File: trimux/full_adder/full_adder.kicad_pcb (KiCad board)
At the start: 2 copper layers, 90.8 x 105.4 mm, 44 parts, among them P1 CONN_01X01, P2 CONN_01X01, P3 CONN_01X01, P4 CONN_01X01, P5 CONN_01X01, P6 CONN_01X03, U1 trimux, U2 trimux, U3 trimux, U4 trimux, U5 trimux, U6 trimux, U7 trimux

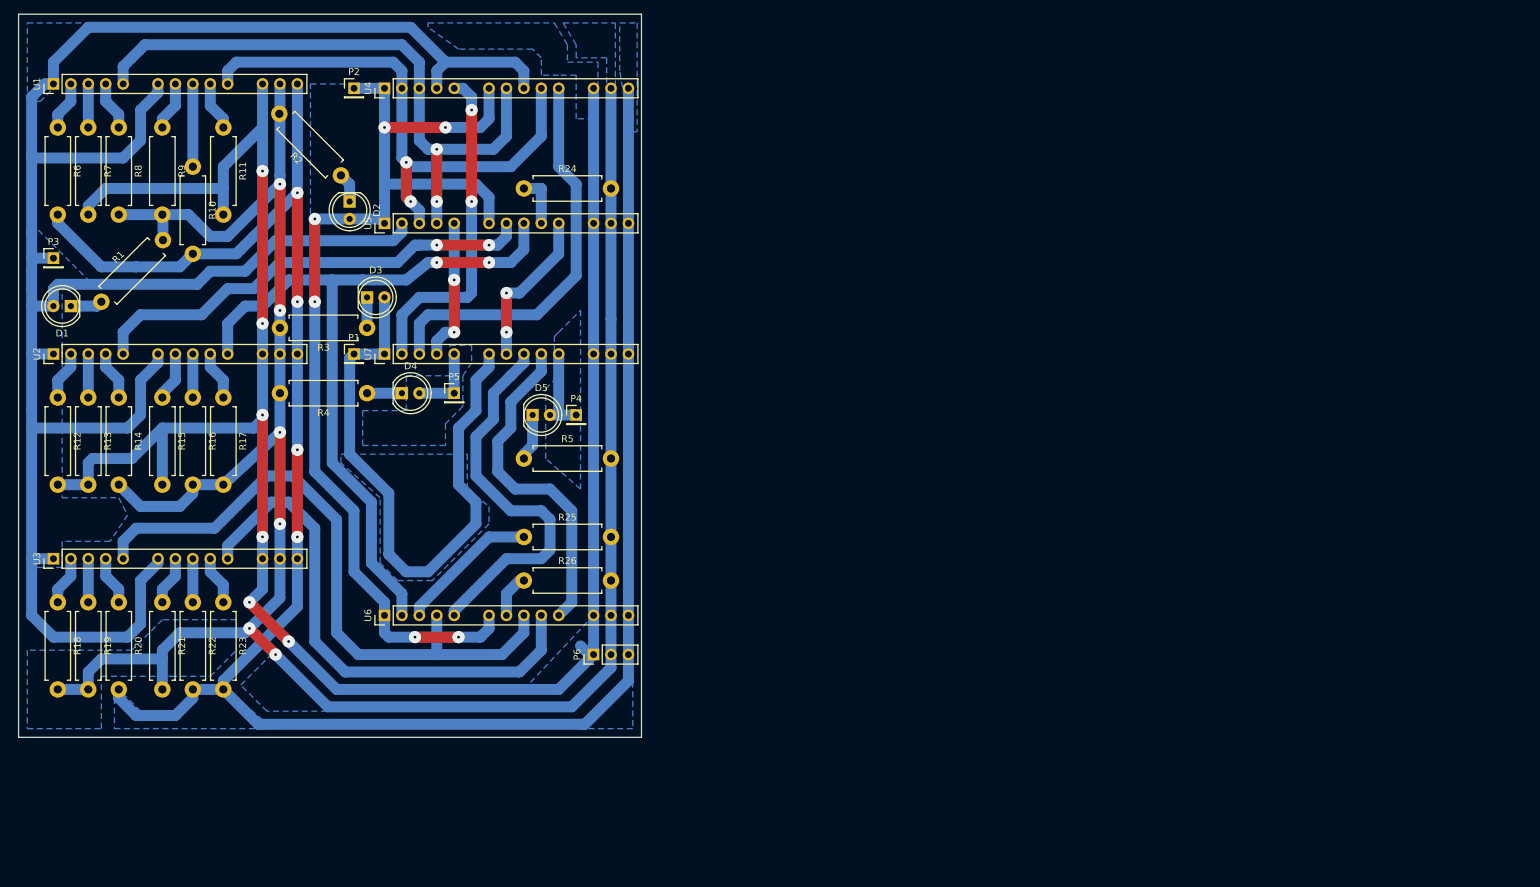
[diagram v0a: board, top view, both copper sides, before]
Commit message: gna
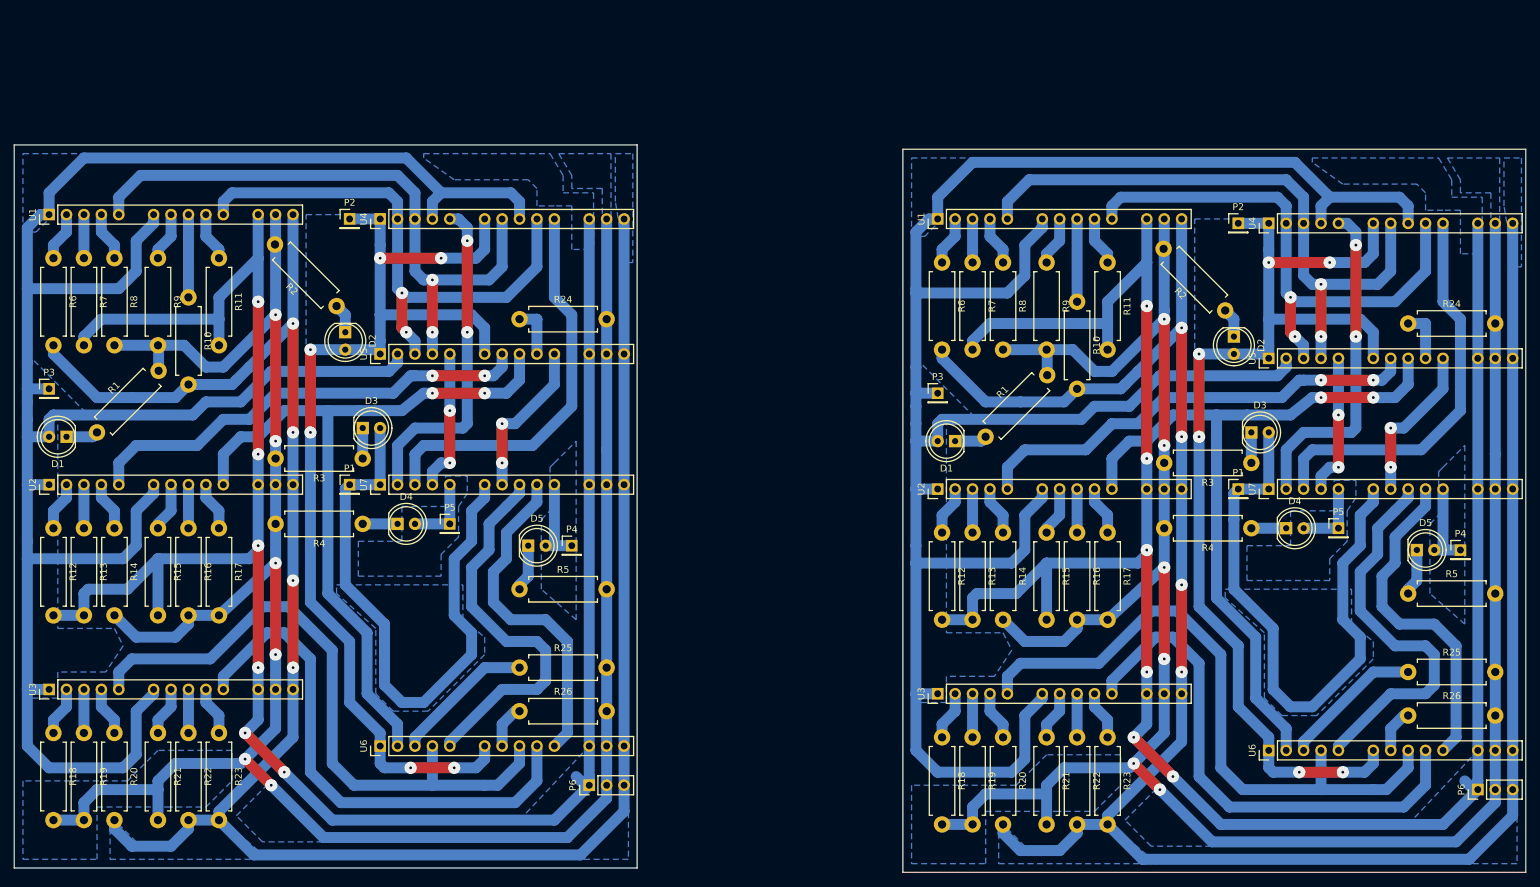
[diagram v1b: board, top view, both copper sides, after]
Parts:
- added D1: LED_Dual_2pin, LEDs:LED_D5.0mm, F.Cu at (177.2, 85.1)
- added D2: LED_Dual_2pin, LEDs:LED_D5.0mm, F.Cu at (217.8, 69.8)
- added D3: LED_Dual_2pin, LEDs:LED_D5.0mm, F.Cu at (220.3, 83.8)
- added D4: LED_Dual_2pin, LEDs:LED_D5.0mm, F.Cu at (225.4, 97.8)
- added D5: LED_Dual_2pin, LEDs:LED_D5.0mm, F.Cu at (244.5, 101.0)
- added P1: CONN_01X01, Pin_Headers:Pin_Header_Straight_1x01_Pitch2.54mm, F.Cu at (218.4, 92.1)
- added P2: CONN_01X01, Pin_Headers:Pin_Header_Straight_1x01_Pitch2.54mm, F.Cu at (218.4, 53.3)
- added P3: CONN_01X01, Pin_Headers:Pin_Header_Straight_1x01_Pitch2.54mm, F.Cu at (174.6, 78.1)
- added P4: CONN_01X01, Pin_Headers:Pin_Header_Straight_1x01_Pitch2.54mm, F.Cu at (250.8, 101.0)
- added P5: CONN_01X01, Pin_Headers:Pin_Header_Straight_1x01_Pitch2.54mm, F.Cu at (233.0, 97.8)
- added P6: CONN_01X03, Pin_Headers:Pin_Header_Straight_1x03_Pitch2.54mm, F.Cu at (253.4, 135.9)
- added R1: 1k, Resistors_THT:R_Axial_DIN0411_L9.9mm_D3.6mm_P12.70mm_Horizontal, F.Cu at (181.6, 84.5)
- added R10: 150, Resistors_THT:R_Axial_DIN0411_L9.9mm_D3.6mm_P12.70mm_Horizontal, F.Cu at (194.9, 64.8)
- added R11: 150, Resistors_THT:R_Axial_DIN0411_L9.9mm_D3.6mm_P12.70mm_Horizontal, F.Cu at (199.4, 59.1)
- added R12: 150, Resistors_THT:R_Axial_DIN0411_L9.9mm_D3.6mm_P12.70mm_Horizontal, F.Cu at (175.3, 98.4)
- added R13: 150, Resistors_THT:R_Axial_DIN0411_L9.9mm_D3.6mm_P12.70mm_Horizontal, F.Cu at (179.7, 98.4)
- added R14: 150, Resistors_THT:R_Axial_DIN0411_L9.9mm_D3.6mm_P12.70mm_Horizontal, F.Cu at (184.2, 98.4)
- added R15: 150, Resistors_THT:R_Axial_DIN0411_L9.9mm_D3.6mm_P12.70mm_Horizontal, F.Cu at (190.5, 98.4)
- added R16: 150, Resistors_THT:R_Axial_DIN0411_L9.9mm_D3.6mm_P12.70mm_Horizontal, F.Cu at (194.9, 98.4)
- added R17: 150, Resistors_THT:R_Axial_DIN0411_L9.9mm_D3.6mm_P12.70mm_Horizontal, F.Cu at (199.4, 98.4)
- added R18: 150, Resistors_THT:R_Axial_DIN0411_L9.9mm_D3.6mm_P12.70mm_Horizontal, F.Cu at (175.3, 128.3)
- added R19: 150, Resistors_THT:R_Axial_DIN0411_L9.9mm_D3.6mm_P12.70mm_Horizontal, F.Cu at (179.7, 128.3)
- added R2: 1k, Resistors_THT:R_Axial_DIN0411_L9.9mm_D3.6mm_P12.70mm_Horizontal, F.Cu at (216.5, 66.0)
- added R20: 150, Resistors_THT:R_Axial_DIN0411_L9.9mm_D3.6mm_P12.70mm_Horizontal, F.Cu at (184.2, 128.3)
- added R21: 150, Resistors_THT:R_Axial_DIN0411_L9.9mm_D3.6mm_P12.70mm_Horizontal, F.Cu at (190.5, 128.3)
- added R22: 150, Resistors_THT:R_Axial_DIN0411_L9.9mm_D3.6mm_P12.70mm_Horizontal, F.Cu at (194.9, 128.3)
- added R23: 150, Resistors_THT:R_Axial_DIN0411_L9.9mm_D3.6mm_P12.70mm_Horizontal, F.Cu at (199.4, 128.3)
- added R24: 150, Resistors_THT:R_Axial_DIN0411_L9.9mm_D3.6mm_P12.70mm_Horizontal, F.Cu at (243.2, 67.9)
- added R25: 150, Resistors_THT:R_Axial_DIN0411_L9.9mm_D3.6mm_P12.70mm_Horizontal, F.Cu at (243.2, 118.7)
- added R26: 150, Resistors_THT:R_Axial_DIN0411_L9.9mm_D3.6mm_P12.70mm_Horizontal, F.Cu at (243.2, 125.1)
- added R3: 1k, Resistors_THT:R_Axial_DIN0411_L9.9mm_D3.6mm_P12.70mm_Horizontal, F.Cu at (220.3, 88.3)
- added R4: 1k, Resistors_THT:R_Axial_DIN0411_L9.9mm_D3.6mm_P12.70mm_Horizontal, F.Cu at (220.3, 97.8)
- added R5: 1k, Resistors_THT:R_Axial_DIN0411_L9.9mm_D3.6mm_P12.70mm_Horizontal, F.Cu at (243.2, 107.3)
- added R6: 150, Resistors_THT:R_Axial_DIN0411_L9.9mm_D3.6mm_P12.70mm_Horizontal, F.Cu at (175.3, 59.1)
- added R7: 150, Resistors_THT:R_Axial_DIN0411_L9.9mm_D3.6mm_P12.70mm_Horizontal, F.Cu at (179.7, 59.1)
- added R8: 150, Resistors_THT:R_Axial_DIN0411_L9.9mm_D3.6mm_P12.70mm_Horizontal, F.Cu at (184.2, 59.1)
- added R9: 150, Resistors_THT:R_Axial_DIN0411_L9.9mm_D3.6mm_P12.70mm_Horizontal, F.Cu at (190.5, 59.1)
- added U1: trimux, trimux:trimux1x15_2.54, F.Cu at (174.6, 52.7)
- added U2: trimux, trimux:trimux1x15_2.54, F.Cu at (174.6, 92.1)
- added U3: trimux, trimux:trimux1x15_2.54, F.Cu at (174.6, 121.9)
- added U4: trimux, trimux:trimux1x15_2.54, F.Cu at (222.9, 53.3)
- added U5: trimux, trimux:trimux1x15_2.54, F.Cu at (222.9, 73.0)
- added U6: trimux, trimux:trimux1x15_2.54, F.Cu at (222.9, 130.2)
- added U7: trimux, trimux:trimux1x15_2.54, F.Cu at (222.9, 92.1)
- moved R12 19.1 mm to (45.7, 97.8)
- moved R13 19.1 mm to (50.2, 97.8)
- moved R14 19.1 mm to (54.6, 97.8)
- moved R15 19.1 mm to (61.0, 97.8)
- moved R16 19.1 mm to (65.4, 97.8)
- moved R17 19.1 mm to (69.8, 97.8)
- moved R18 19.1 mm to (45.7, 127.6)
- moved R19 19.1 mm to (50.2, 127.6)
- moved R20 19.1 mm to (54.6, 127.6)
- moved R21 19.1 mm to (61.0, 127.6)
- moved R22 19.1 mm to (65.4, 127.6)
- moved R23 19.1 mm to (69.8, 127.6)
- moved R5 19.1 mm to (113.7, 106.7)
- moved D2 19.1 mm to (88.3, 69.2)
- moved R10 19.1 mm to (65.4, 64.1)
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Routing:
- net GNDREF: track 325.3 -> 650.7 mm, vias 6 -> 12
- net /A: track 315.0 -> 630.0 mm
- net +5V: track 306.1 -> 612.1 mm, vias 4 -> 8
- net -5V: track 300.5 -> 601.0 mm, vias 6 -> 12
- net /B: track 157.1 -> 314.1 mm, vias 6 -> 12
- net /min(A,0): track 108.8 -> 217.7 mm, vias 2 -> 4
- net /max(A.0): track 94.9 -> 189.9 mm
- net /A-1: track 91.3 -> 182.6 mm, vias 2 -> 4
- net /Cin: track 89.7 -> 179.5 mm
- net /A+1: track 80.4 -> 160.8 mm, vias 2 -> 4
- net /min(A,0)+1: track 76.6 -> 153.2 mm
- net /max(A,0)-1: track 66.7 -> 133.5 mm, vias 2 -> 4
- net /B+A: track 58.6 -> 117.1 mm
- net Net-(U6-Pad5): track 56.8 -> 113.7 mm
- net Net-(U6-Pad11): track 49.0 -> 97.9 mm
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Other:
- board size 90.8 x 105.4 mm -> 220.3 x 106 mm
